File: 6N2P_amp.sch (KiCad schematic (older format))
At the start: 79 parts, among them J1 guitar_in, J2 speaker, J3 fx_send, J4 fx_return, J5 foot_sw, U1 ECC83, U2 ECC83, U3 6N1P, U4 DSN-MINI-360, U5 DSN-MINI-360, U6 DSN-MINI-360, U7 NCH6100HV

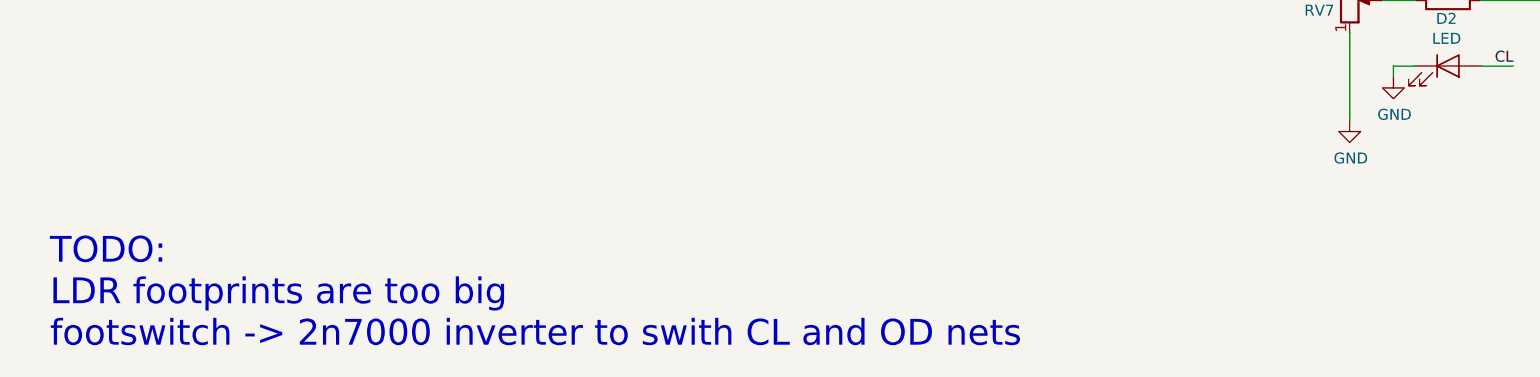
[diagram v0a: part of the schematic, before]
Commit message: genug fuer heute
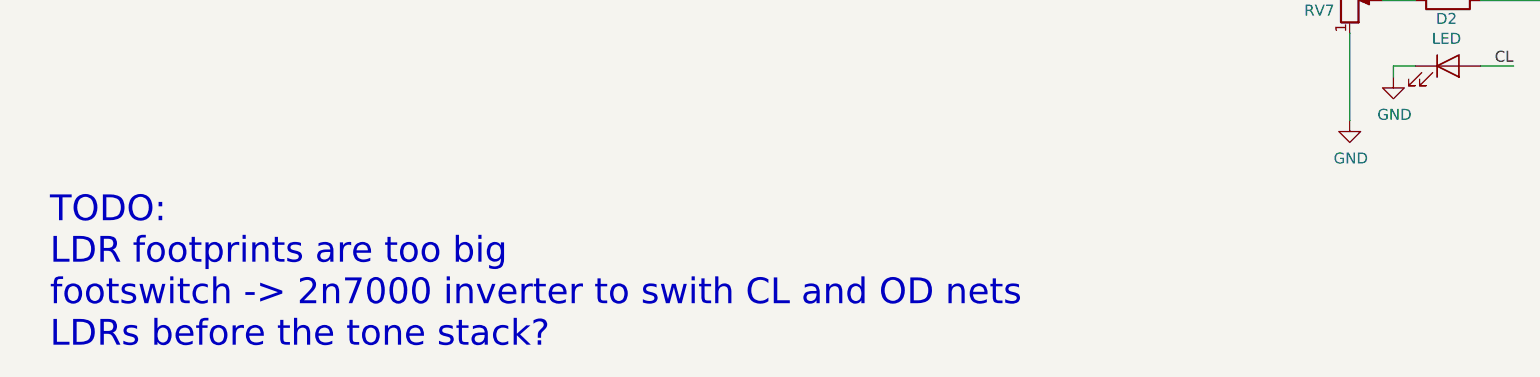
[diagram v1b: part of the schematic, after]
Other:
- note added: "TODO:\nLDR footprints are too big\nfootswitch -> 2n7000 inverter to swith CL and OD nets\nLDRs before the tone stack?"
- note removed: "TODO:\nLDR footprints are too big\nfootswitch -> 2n7000 inverter to swith CL and OD nets"
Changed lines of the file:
@@
 	12900 8500 12900 8450
 Text Notes 1550 13600 0    118  ~ 0
-TODO:\nLDR footprints are too big\nfootswitch -> 2n7000 inverter to swith CL and OD nets
+TODO:\nLDR footprints are too big\nfootswitch -> 2n7000 inverter to swith CL and OD nets\nLDRs before the tone stack?
 $Comp
 L micha_custom:6.3MMTRSSwitched J5
